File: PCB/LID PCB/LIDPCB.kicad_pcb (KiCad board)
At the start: 2 copper layers, 22 x 17 mm, 10 parts, among them J1 POWER/I2C, U1 LTR-329ALS-01, U2 LSM6DSMTR

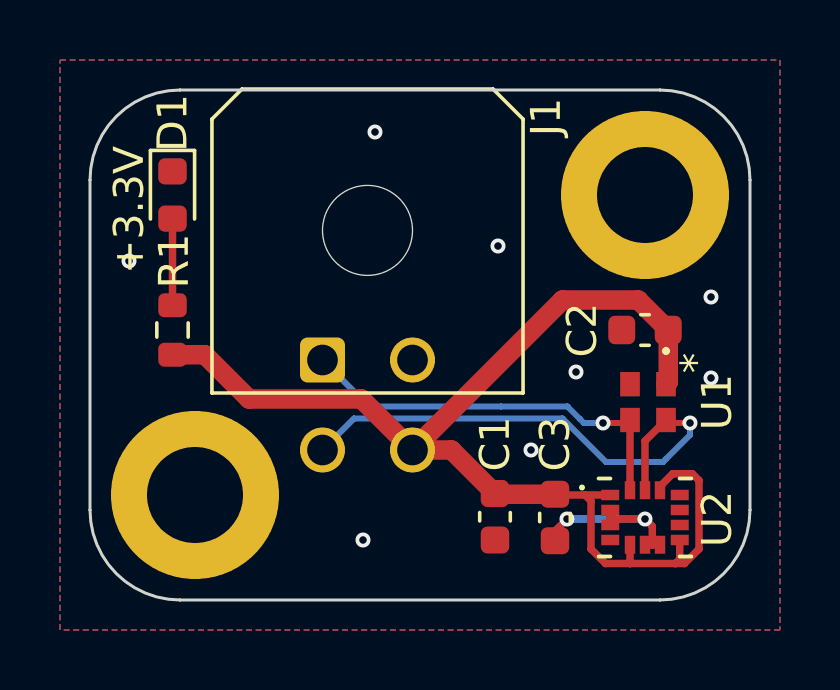
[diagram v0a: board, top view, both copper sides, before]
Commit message: Main pcb reviewed
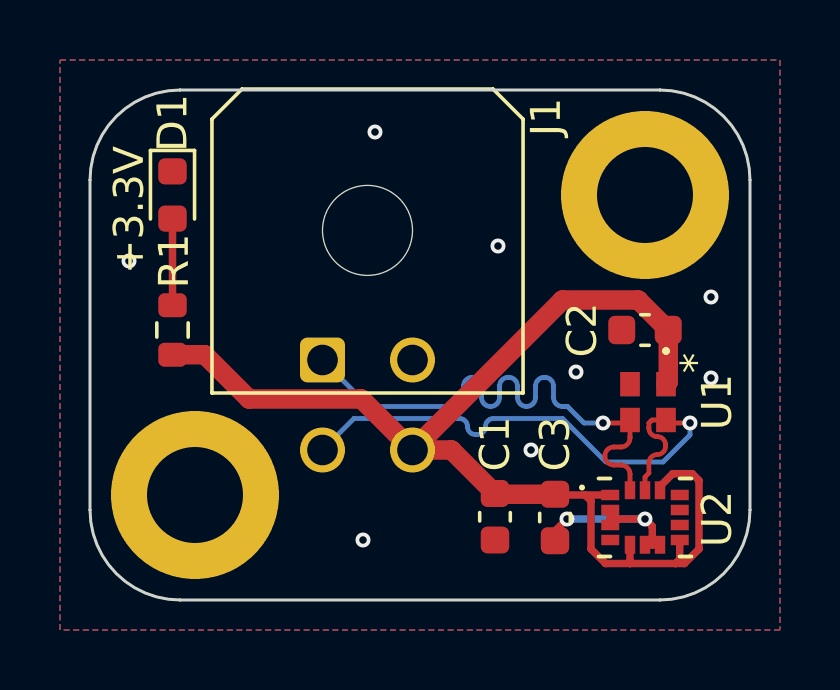
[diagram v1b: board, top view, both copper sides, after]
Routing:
- net /SDA: track 13.5 -> 18.8 mm
- net /SCL: track 17.5 -> 19.0 mm
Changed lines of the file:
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@@
   (segment (start 115.9 114.3) (end 118.5 114.3) (width 0.25) (layer "B.Cu") (net 2))
   (segment (start 102.75 107.175) (end 102.75 104.2875) (width 0.25) (layer "F.Cu") (net 3))
-  (segment (start 117.1 111.1) (end 117.9 111.1) (width 0.2) (layer "F.Cu") (net 4))
-  (segment (start 117.9 111.1) (end 118 111) (width 0.2) (layer "F.Cu") (net 4))
-  (segment (start 118 111) (end 118 113.34) (width 0.25) (layer "F.Cu") (net 4))
+  (segment (start 118 113.34) (end 118 112.8) (width 0.16) (layer "F.Cu") (net 4))
+  (segment (start 117.1 111.1) (end 117.9 111.1) (width 0.16) (layer "F.Cu") (net 4))
+  (segment (start 117.462476 111.9) (end 117.7 111.9) (width 0.16) (layer "F.Cu") (net 4))
+  (segment (start 117.9 111.1) (end 118 111) (width 0.16) (layer "F.Cu") (net 4))
+  (segment (start 118 111.6) (end 118 111.55) (width 0.16) (layer "F.Cu") (net 4))
+  (segment (start 117.7 112.5) (end 117.462476 112.5) (width 0.16) (layer "F.Cu") (net 4))
+  (segment (start 118 111.55) (end 118 111) (width 0.16) (layer "F.Cu") (net 4))
   (via (at 117.1 111.1) (size 0.5) (drill 0.25) (layers "F.Cu" "B.Cu") (net 4))
-  (segment (start 107.75 109) (end 109.3 110.55) (width 0.2) (layer "B.Cu") (net 4))
-  (segment (start 109.3 110.55) (end 113.7 110.55) (width 0.2) (layer "B.Cu") (net 4))
-  (segment (start 115.915686 110.55) (end 116.332843 110.967157) (width 0.2) (layer "B.Cu") (net 4))
-  (segment (start 116.465686 111.1) (end 117.1 111.1) (width 0.2) (layer "B.Cu") (net 4))
-  (segment (start 116.332843 110.967157) (end 116.465686 111.1) (width 0.2) (layer "B.Cu") (net 4))
-  (segment (start 113.7 110.55) (end 115.915686 110.55) (width 0.2) (layer "B.Cu") (net 4))
-  (segment (start 118.5 111.699998) (end 118.5 113.34) (width 0.25) (layer "F.Cu") (net 5))
-  (segment (start 119.299998 111.1) (end 119.199998 111) (width 0.2) (layer "F.Cu") (net 5))
-  (segment (start 119.199998 111) (end 118.5 111.699998) (width 0.25) (layer "F.Cu") (net 5))
-  (segment (start 120 111.1) (end 119.299998 111.1) (width 0.2) (layer "F.Cu") (net 5))
+  (arc (start 117.162476 112.2) (mid 117.250344 111.987868) (end 117.462476 111.9) (width 0.16) (layer "F.Cu") (net 4))
+  (arc (start 117.462476 112.5) (mid 117.250344 112.412132) (end 117.162476 112.2) (width 0.16) (layer "F.Cu") (net 4))
+  (arc (start 117.7 111.9) (mid 117.912132 111.812132) (end 118 111.6) (width 0.16) (layer "F.Cu") (net 4))
+  (arc (start 118 112.8) (mid 117.912132 112.587868) (end 117.7 112.5) (width 0.16) (layer "F.Cu") (net 4))
+  (segment (start 115.75 110.55) (end 115.8 110.55) (width 0.16) (layer "B.Cu") (net 4))
+  (segment (start 114.25 109.876854) (end 114.25 110.25) (width 0.16) (layer "B.Cu") (net 4))
+  (segment (start 114.85 110.25) (end 114.85 109.876854) (width 0.16) (layer "B.Cu") (net 4))
+  (segment (start 115.915686 110.55) (end 116.465686 111.1) (width 0.16) (layer "B.Cu") (net 4))
+  (segment (start 116.465686 111.1) (end 117.1 111.1) (width 0.16) (layer "B.Cu") (net 4))
+  (segment (start 115.8 110.55) (end 115.915686 110.55) (width 0.16) (layer "B.Cu") (net 4))
+  (segment (start 115.45 109.876854) (end 115.45 110.25) (width 0.16) (layer "B.Cu") (net 4))
+  (segment (start 107.75 109) (end 109.3 110.55) (width 0.16) (layer "B.Cu") (net 4))
+  (segment (start 109.3 110.55) (end 112.15 110.55) (width 0.16) (layer "B.Cu") (net 4))
+  (segment (start 113.05 109.876854) (end 113.05 110.25) (width 0.16) (layer "B.Cu") (net 4))
+  (segment (start 112.45 110.25) (end 112.45 109.876854) (width 0.16) (layer "B.Cu") (net 4))
+  (segment (start 113.65 110.25) (end 113.65 109.876854) (width 0.16) (layer "B.Cu") (net 4))
+  (arc (start 114.85 109.876854) (mid 114.937868 109.664722) (end 115.15 109.576854) (width 0.16) (layer "B.Cu") (net 4))
+  (arc (start 114.25 110.25) (mid 114.337868 110.462132) (end 114.55 110.55) (width 0.16) (layer "B.Cu") (net 4))
+  (arc (start 115.45 110.25) (mid 115.537868 110.462132) (end 115.75 110.55) (width 0.16) (layer "B.Cu") (net 4))
+  (arc (start 113.95 109.576854) (mid 114.162132 109.664722) (end 114.25 109.876854) (width 0.16) (layer "B.Cu") (net 4))
+  (arc (start 112.15 110.55) (mid 112.362132 110.462132) (end 112.45 110.25) (width 0.16) (layer "B.Cu") (net 4))
+  (arc (start 113.65 109.876854) (mid 113.737868 109.664722) (end 113.95 109.576854) (width 0.16) (layer "B.Cu") (net 4))
+  (arc (start 112.75 109.576854) (mid 112.962132 109.664722) (end 113.05 109.876854) (width 0.16) (layer "B.Cu") (net 4))
+  (arc (start 112.45 109.876854) (mid 112.537868 109.664722) (end 112.75 109.576854) (width 0.16) (layer "B.Cu") (net 4))
+  (arc (start 113.05 110.25) (mid 113.137868 110.462132) (end 113.35 110.55) (width 0.16) (layer "B.Cu") (net 4))
+  (arc (start 115.15 109.576854) (mid 115.362132 109.664722) (end 115.45 109.876854) (width 0.16) (layer "B.Cu") (net 4))
+  (arc (start 113.35 110.55) (mid 113.562132 110.462132) (end 113.65 110.25) (width 0.16) (layer "B.Cu") (net 4))
+  (arc (start 114.55 110.55) (mid 114.762132 110.462132) (end 114.85 110.25) (width 0.16) (layer "B.Cu") (net 4))
+  (segment (start 118.5 112.9) (end 118.6302 112.7698) (width 0.16) (layer "F.Cu") (net 5))
+  (segment (start 118.6302 112.7698) (end 118.6302 112.4302) (width 0.16) (layer "F.Cu") (net 5))
+  (segment (start 118.7302 111) (end 119.199998 111) (width 0.16) (layer "F.Cu") (net 5))
+  (segment (start 118.6302 111.1) (end 118.7302 111) (width 0.16) (layer "F.Cu") (net 5))
+  (segment (start 119.299998 111.1) (end 119.199998 111) (width 0.16) (layer "F.Cu") (net 5))
+  (segment (start 118.6302 111.2302) (end 118.6302 111.1) (width 0.16) (layer "F.Cu") (net 5))
+  (segment (start 119.18515 111.87525) (end 119.18515 111.8302) (width 0.16) (layer "F.Cu") (net 5))
+  (segment (start 118.6302 111.27525) (end 118.6302 111.2302) (width 0.16) (layer "F.Cu") (net 5))
+  (segment (start 120 111.1) (end 119.299998 111.1) (width 0.16) (layer "F.Cu") (net 5))
+  (segment (start 118.5 113.34) (end 118.5 112.9) (width 0.16) (layer "F.Cu") (net 5))
   (via (at 120 111.1) (size 0.5) (drill 0.25) (layers "F.Cu" "B.Cu") (net 5))
-  (segment (start 107.75 112) (end 108.8 110.95) (width 0.2) (layer "B.Cu") (net 5))
-  (segment (start 120 111.2) (end 120 111.1) (width 0.2) (layer "B.Cu") (net 5))
-  (segment (start 119.2 112.3) (end 120 111.5) (width 0.2) (layer "B.Cu") (net 5))
-  (segment (start 117.2 112.4) (end 119.1 112.4) (width 0.2) (layer "B.Cu") (net 5))
-  (segment (start 119.1 112.4) (end 119.2 112.3) (width 0.2) (layer "B.Cu") (net 5))
-  (segment (start 120 111.5) (end 120 111.2) (width 0.2) (layer "B.Cu") (net 5))
-  (segment (start 108.8 110.95) (end 115.75 110.95) (width 0.2) (layer "B.Cu") (net 5))
-  (segment (start 115.75 110.95) (end 117.2 112.4) (width 0.2) (layer "B.Cu") (net 5))
+  (arc (start 118.907675 112.152725) (mid 119.103879 112.071454) (end 119.18515 111.87525) (width 0.16) (layer "F.Cu") (net 5))
+  (arc (start 118.6302 112.4302) (mid 118.711471 112.233996) (end 118.907675 112.152725) (width 0.16) (layer "F.Cu") (net 5))
+  (arc (start 119.18515 111.8302) (mid 119.103879 111.633996) (end 118.907675 111.552725) (width 0.16) (layer "F.Cu") (net 5))
+  (arc (start 118.907675 111.552725) (mid 118.711471 111.471454) (end 118.6302 111.27525) (width 0.16) (layer "F.Cu") (net 5))
+  (segment (start 119.1 112.4) (end 117.2 112.4) (width 0.16) (layer "B.Cu") (net 5))
+  (segment (start 117.2 112.4) (end 115.75 110.95) (width 0.16) (layer "B.Cu") (net 5))
+  (segment (start 112.91485 111.485151) (end 112.85 111.485151) (width 0.16) (layer "B.Cu") (net 5))
+  (segment (start 108.8 110.95) (end 107.75 112) (width 0.16) (layer "B.Cu") (net 5))
+  (segment (start 115.75 110.95) (end 113.45 110.95) (width 0.16) (layer "B.Cu") (net 5))
+  (segment (start 112.25 110.95) (end 108.8 110.95) (width 0.16) (layer "B.Cu") (net 5))
+  (segment (start 112.582425 111.217576) (end 112.582425 111.217575) (width 0.16) (layer "B.Cu") (net 5))
+  (segment (start 113.182425 111.217575) (end 113.182425 111.217576) (width 0.16) (layer "B.Cu") (net 5))
+  (segment (start 112.31485 110.95) (end 112.25 110.95) (width 0.16) (layer "B.Cu") (net 5))
+  (segment (start 120 111.5) (end 119.1 112.4) (width 0.16) (layer "B.Cu") (net 5))
+  (segment (start 120 111.1) (end 120 111.5) (width 0.16) (layer "B.Cu") (net 5))
+  (arc (start 112.85 111.485151) (mid 112.660796 111.40678) (end 112.582425 111.217576) (width 0.16) (layer "B.Cu") (net 5))
+  (arc (start 112.582425 111.217575) (mid 112.504054 111.028371) (end 112.31485 110.95) (width 0.16) (layer "B.Cu") (net 5))
+  (arc (start 113.182425 111.217576) (mid 113.104054 111.40678) (end 112.91485 111.485151) (width 0.16) (layer "B.Cu") (net 5))
+  (arc (start 113.45 110.95) (mid 113.260796 111.028371) (end 113.182425 111.217575) (width 0.16) (layer "B.Cu") (net 5))
   (zone (net 2) (net_name "GND") (layers F&B.Cu) (hatch edge 0.508)
     (priority 1)
